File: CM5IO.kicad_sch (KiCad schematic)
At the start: 18 parts, among them J11 USB_C_Receptacle_USB2.0, J4 ATX-24, Q1 MMBT7002K, Q2 DMP3013SFV-7

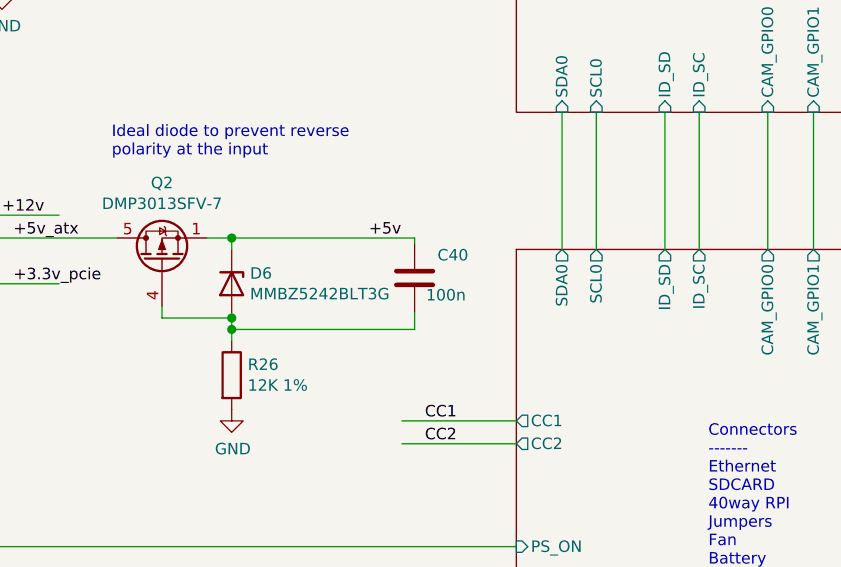
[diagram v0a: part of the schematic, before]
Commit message: more aisler changes
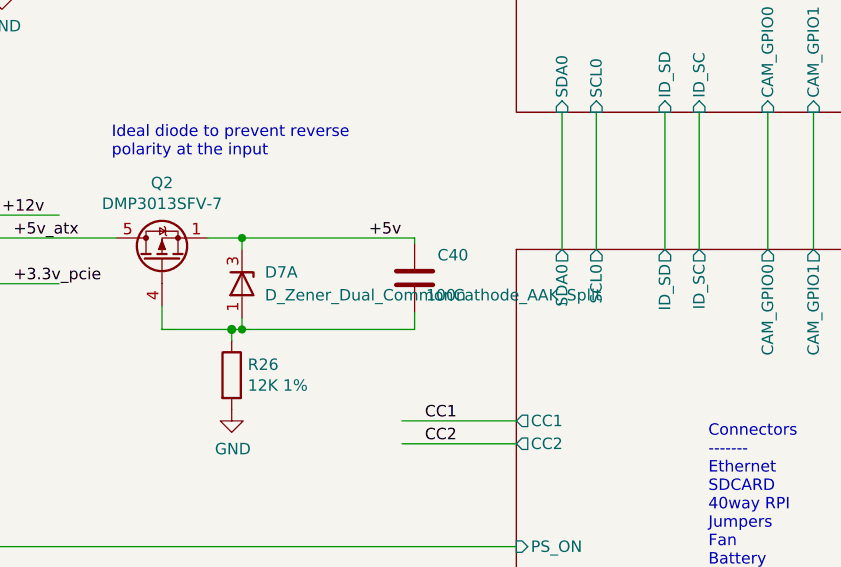
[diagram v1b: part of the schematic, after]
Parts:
- removed D6: MMBZ5242BLT3G, Diode_SMD:D_SOT-23_ANK, symbol Diode:BZX84Cxx
- added D7: D_Zener_Dual_CommonCathode_AAK_Split, Package_TO_SOT_SMD:SOT-23, symbol Device:D_Zener_Dual_CommonCathode_AAK_Split
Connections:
- net +5v: now also D7.3 (K)
- net at C40.2, Q2.4 (G), R26.1: now also D7.1 (A)
